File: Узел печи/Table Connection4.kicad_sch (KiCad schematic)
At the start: 0 parts

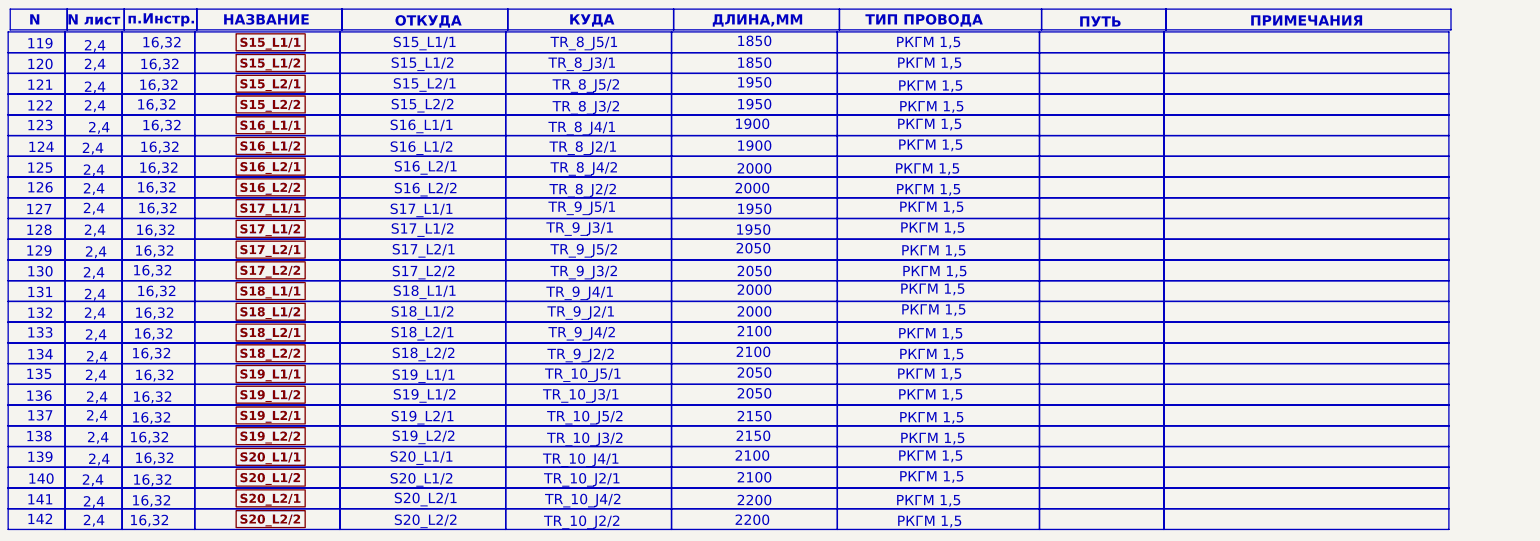
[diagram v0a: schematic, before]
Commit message: update schemas
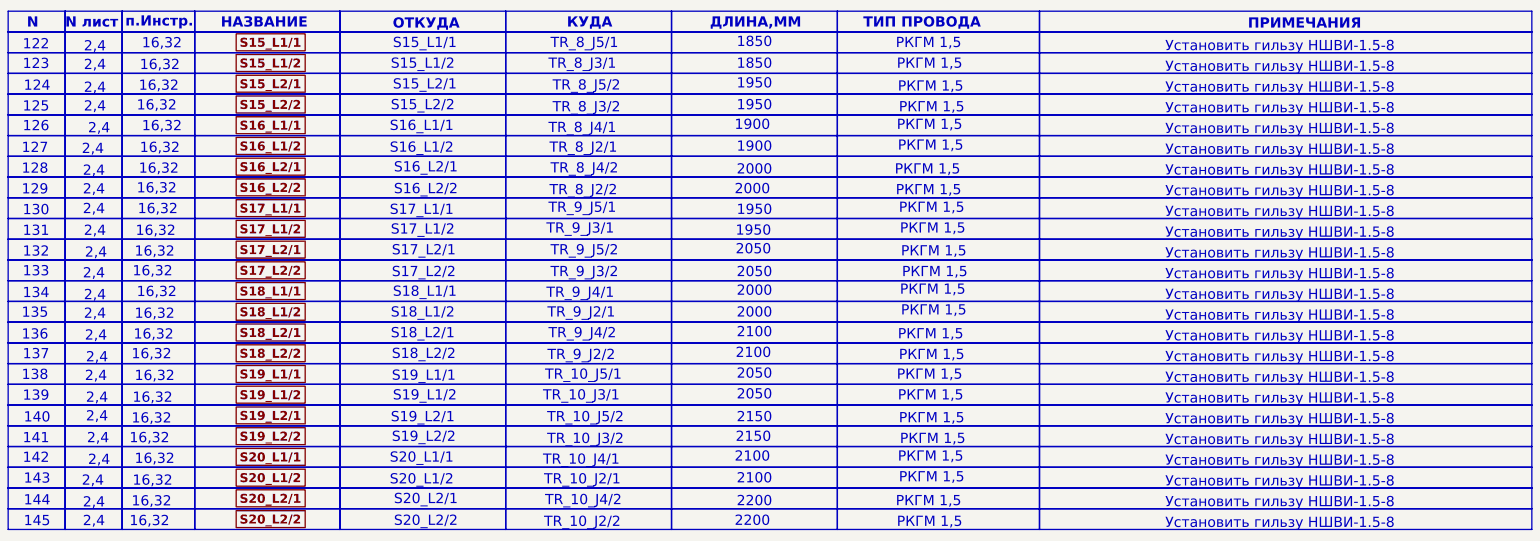
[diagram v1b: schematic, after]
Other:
- note added: "143"
- note added: "144"
- note added: "145"
- note added: "Установить гильзу НШВИ-1.5-8"
- note removed: "119"
- note removed: "120"
- note removed: "121"
- note removed: "ПУТЬ"
